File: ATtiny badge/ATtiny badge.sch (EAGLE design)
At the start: 4 parts, among them IC1 TINY13-20SSU

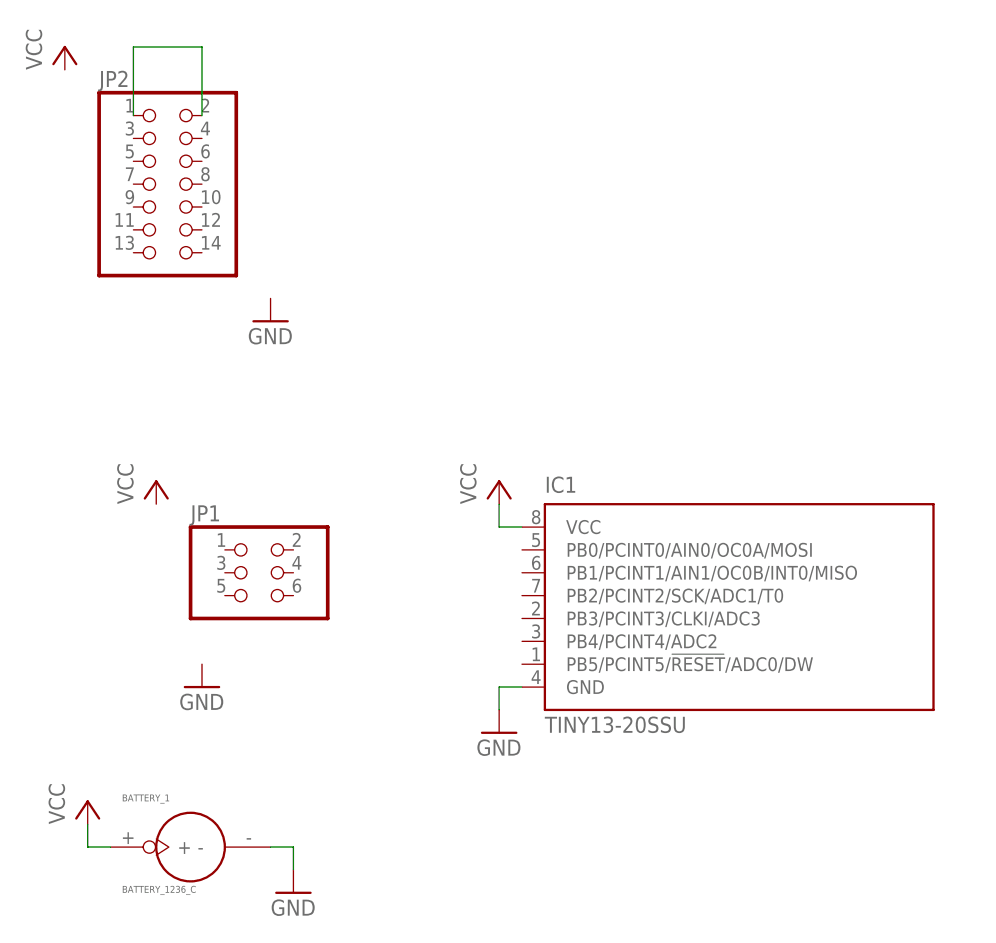
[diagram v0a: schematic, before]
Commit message: new badges
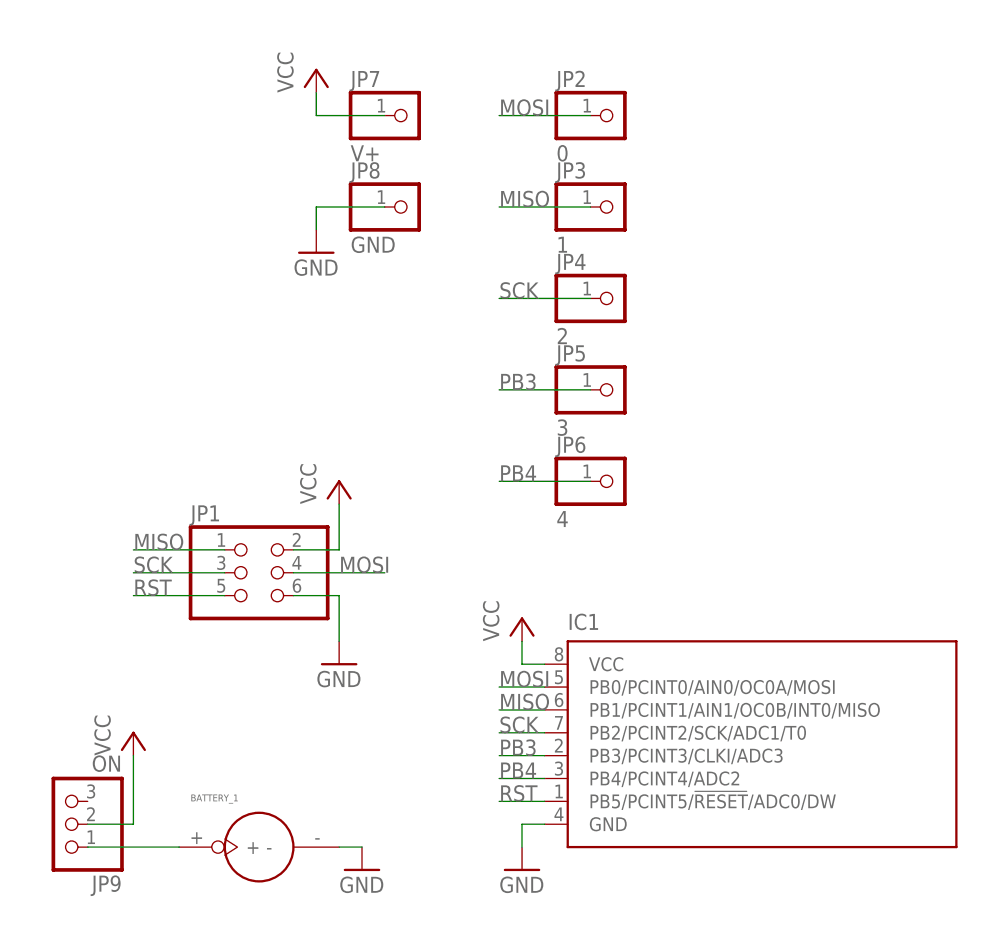
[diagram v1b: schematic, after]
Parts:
- added JP3: 1, pinhead:PINHD-1X1
- added JP4: 2, pinhead:PINHD-1X1
- added JP5: 3, pinhead:PINHD-1X1
- added JP6: 4, pinhead:PINHD-1X1
- added JP7: V+, pinhead:PINHD-1X1
- added JP8: GND, pinhead:PINHD-1X1
- added JP9: ON, pinhead:PINHD-1X3
- IC1: value TINY13-20SSU -> TINY13-20SU; device atmel:TINY13-20SSU -> atmel:TINY13-20SU
- JP2: value (none) -> 0; device pinhead:PINHD-2X7 -> pinhead:PINHD-1X1
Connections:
- new net MISO: IC1.PB1/PCINT1/AIN1/OC0B/INT0/MISO, JP1.1, JP3.1
- new net MOSI: IC1.PB0/PCINT0/AIN0/OC0A/MOSI, JP1.4, JP2.1
- new net PB3: IC1.PB3/PCINT3/CLKI/ADC3, JP5.1
- new net PB4: IC1.PB4/PCINT4/ADC2, JP6.1
- new net RST: IC1.PB5/PCINT5/!RESET!/ADC0/DW, JP1.5
- new net SCK: IC1.PB2/PCINT2/SCK/ADC1/T0, JP1.3, JP4.1
- net GND: now also JP1.6, JP8.1
- net N$1: now also BATTERY_1.+, JP9.1; no longer JP2.1, JP2.2
- net VCC: now also JP1.2, JP7.1, JP9.2; no longer BATTERY_1.+
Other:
- moved on the sheet: BATTERY_1, IC1
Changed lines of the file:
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@@
 </classes>
 <parts>
-<part name="BATTERY_1" library="Itead_BP_110825.lbr" deviceset="BATTERY_1236_C" device=""/>
-<part name="IC1" library="atmel" deviceset="TINY13" device="SSU" technology="-20"/>
+<part name="BATTERY_1" library="Itead_BP_110825.lbr" deviceset="BATTERY_1236_C" device="" value=""/>
+<part name="IC1" library="atmel" deviceset="TINY13" device="SU" technology="-20" value=""/>
 <part name="JP1" library="pinhead" deviceset="PINHD-2X3" device=""/>
-<part name="JP2" library="pinhead" deviceset="PINHD-2X7" device=""/>
 <part name="GND1" library="supply1" deviceset="GND" device=""/>
 <part name="GND2" library="supply1" deviceset="GND" device=""/>
@@
 <part name="P+3" library="supply1" deviceset="VCC" device=""/>
 <part name="P+4" library="supply1" deviceset="VCC" device=""/>
+<part name="JP2" library="pinhead" deviceset="PINHD-1X1" device="" value="0  "/>
+<part name="JP3" library="pinhead" deviceset="PINHD-1X1" device="" value="1  "/>
+<part name="JP4" library="pinhead" deviceset="PINHD-1X1" device="" value="2  "/>
+<part name="JP5" library="pinhead" deviceset="PINHD-1X1" device="" value="3  "/>
+<part name="JP6" library="pinhead" deviceset="PINHD-1X1" device="" value="4  "/>
+<part name="JP7" library="pinhead" deviceset="PINHD-1X1" device="" value="V+"/>
+<part name="JP8" library="pinhead" deviceset="PINHD-1X1" device="" value="GND"/>
+<part name="JP9" library="pinhead" deviceset="PINHD-1X3" device="" value="ON"/>
 </parts>
 <sheets>
@@
 </plain>
 <instances>
-<instance part="BATTERY_1" gate="G$1" x="16.51" y="7.62"/>
-<instance part="IC1" gate="G$1" x="73.66" y="30.48"/>
+<instance part="BATTERY_1" gate="G$1" x="24.13" y="7.62"/>
+<instance part="IC1" gate="G$1" x="76.2" y="15.24"/>
 <instance part="JP1" gate="A" x="22.86" y="38.1"/>
-<instance part="JP2" gate="A" x="12.7" y="81.28"/>
-<instance part="GND1" gate="1" x="27.94" y="2.54"/>
-<instance part="GND2" gate="1" x="50.8" y="20.32"/>
-<instance part="GND3" gate="1" x="25.4" y="66.04"/>
-<instance part="GND4" gate="1" x="17.78" y="25.4"/>
-<instance part="P+1" gate="VCC" x="5.08" y="12.7"/>
-<instance part="P+2" gate="VCC" x="12.7" y="48.26"/>
-<instance part="P+3" gate="VCC" x="50.8" y="48.26"/>
-<instance part="P+4" gate="VCC" x="2.54" y="96.52"/>
+<instance part="GND1" gate="1" x="35.56" y="5.08"/>
+<instance part="GND2" gate="1" x="53.34" y="5.08"/>
+<instance part="GND3" gate="1" x="30.48" y="73.66"/>
+<instance part="GND4" gate="1" x="33.02" y="27.94"/>
+<instance part="P+1" gate="VCC" x="10.16" y="20.32"/>
+<instance part="P+2" gate="VCC" x="33.02" y="48.26"/>
+<instance part="P+3" gate="VCC" x="53.34" y="33.02"/>
+<instance part="P+4" gate="VCC" x="30.48" y="93.98"/>
+<instance part="JP2" gate="G$1" x="63.5" y="88.9"/>
+<instance part="JP3" gate="G$1" x="63.5" y="78.74"/>
+<instance part="JP4" gate="G$1" x="63.5" y="68.58"/>
+<instance part="JP5" gate="G$1" x="63.5" y="58.42"/>
+<instance part="JP6" gate="G$1" x="63.5" y="48.26"/>
+<instance part="JP7" gate="G$1" x="40.64" y="88.9"/>
+<instance part="JP8" gate="G$1" x="40.64" y="78.74"/>
+<instance part="JP9" gate="A" x="2.54" y="10.16" rot="R180"/>
 </instances>
 <busses>
@@
 <pinref part="BATTERY_1" gate="G$1" pin="-"/>
 <pinref part="GND1" gate="1" pin="GND"/>
-<wire x1="25.4" y1="7.62" x2="27.94" y2="7.62" width="0.1524" layer="91"/>
-<wire x1="27.94" y1="7.62" x2="27.94" y2="5.08" width="0.1524" layer="91"/>
+<wire x1="33.02" y1="7.62" x2="35.56" y2="7.62" width="0.1524" layer="91"/>
 </segment>
 <segment>
 <pinref part="IC1" gate="G$1" pin="GND"/>
 <pinref part="GND2" gate="1" pin="GND"/>
-<wire x1="53.34" y1="25.4" x2="50.8" y2="25.4" width="0.1524" layer="91"/>
-<wire x1="50.8" y1="25.4" x2="50.8" y2="22.86" width="0.1524" layer="91"/>
+<wire x1="55.88" y1="10.16" x2="53.34" y2="10.16" width="0.1524" layer="91"/>
+<wire x1="53.34" y1="10.16" x2="53.34" y2="7.62" width="0.1524" layer="91"/>
+</segment>
+<segment>
+<pinref part="GND3" gate="1" pin="GND"/>
+<pinref part="JP8" gate="G$1" pin="1"/>
+<wire x1="30.48" y1="76.2" x2="30.48" y2="78.74" width="0.1524" layer="91"/>
+<wire x1="30.48" y1="78.74" x2="38.1" y2="78.74" width="0.1524" layer="91"/>
+</segment>
+<segment>
+<pinref part="JP1" gate="A" pin="6"/>
+<wire x1="27.94" y1="35.56" x2="33.02" y2="35.56" width="0.1524" layer="91"/>
+<wire x1="33.02" y1="35.56" x2="33.02" y2="30.48" width="0.1524" layer="91"/>
+<pinref part="GND4" gate="1" pin="GND"/>
 </segment>
 </net>
 <net name="VCC" class="0">
 <segment>
-<pinref part="BATTERY_1" gate="G$1" pin="+"/>
-<pinref part="P+1" gate="VCC" pin="VCC"/>
-<wire x1="7.62" y1="7.62" x2="5.08" y2="7.62" width="0.1524" layer="91"/>
-<wire x1="5.08" y1="7.62" x2="5.08" y2="10.16" width="0.1524" layer="91"/>
+<pinref part="IC1" gate="G$1" pin="VCC"/>
+<pinref part="P+3" gate="VCC" pin="VCC"/>
+<wire x1="55.88" y1="27.94" x2="53.34" y2="27.94" width="0.1524" layer="91"/>
+<wire x1="53.34" y1="27.94" x2="53.34" y2="30.48" width="0.1524" layer="91"/>
 </segment>
 <segment>
-<pinref part="IC1" gate="G$1" pin="VCC"/>
-<pinref part="P+3" gate="VCC" pin="VCC"/>
-<wire x1="53.34" y1="43.18" x2="50.8" y2="43.18" width="0.1524" layer="91"/>
-<wire x1="50.8" y1="43.18" x2="50.8" y2="45.72" width="0.1524" layer="91"/>
+<pinref part="P+4" gate="VCC" pin="VCC"/>
+<pinref part="JP7" gate="G$1" pin="1"/>
+<wire x1="30.48" y1="91.44" x2="30.48" y2="88.9" width="0.1524" layer="91"/>
+<wire x1="30.48" y1="88.9" x2="38.1" y2="88.9" width="0.1524" layer="91"/>
+</segment>
+<segment>
+<pinref part="P+2" gate="VCC" pin="VCC"/>
+<wire x1="33.02" y1="45.72" x2="33.02" y2="40.64" width="0.1524" layer="91"/>
+<pinref part="JP1" gate="A" pin="2"/>
+<wire x1="33.02" y1="40.64" x2="27.94" y2="40.64" width="0.1524" layer="91"/>
+</segment>
+<segment>
+<pinref part="JP9" gate="A" pin="2"/>
+<pinref part="P+1" gate="VCC" pin="VCC"/>
+<wire x1="5.08" y1="10.16" x2="10.16" y2="10.16" width="0.1524" layer="91"/>
+<wire x1="10.16" y1="10.16" x2="10.16" y2="17.78" width="0.1524" layer="91"/>
+</segment>
+</net>
+<net name="MISO" class="0">
+<segment>
+<pinref part="JP1" gate="A" pin="1"/>
+<wire x1="20.32" y1="40.64" x2="10.16" y2="40.64" width="0.1524" layer="91"/>
+<label x="10.16" y="40.64" size="1.778" layer="95"/>
+</segment>
+<segment>
+<pinref part="IC1" gate="G$1" pin="PB1/PCINT1/AIN1/OC0B/INT0/MISO"/>
+<wire x1="55.88" y1="22.86" x2="50.8" y2="22.86" width="0.1524" layer="91"/>
+<label x="50.8" y="22.86" size="1.778" layer="95"/>
+</segment>
+<segment>
+<pinref part="JP3" gate="G$1" pin="1"/>
+<wire x1="60.96" y1="78.74" x2="50.8" y2="78.74" width="0.1524" layer="91"/>
+<label x="50.8" y="78.74" size="1.778" layer="95"/>
+</segment>
+</net>
+<net name="SCK" class="0">
+<segment>
+<pinref part="JP1" gate="A" pin="3"/>
+<wire x1="20.32" y1="38.1" x2="10.16" y2="38.1" width="0.1524" layer="91"/>
+<label x="10.16" y="38.1" size="1.778" layer="95"/>
+</segment>
+<segment>
+<pinref part="IC1" gate="G$1" pin="PB2/PCINT2/SCK/ADC1/T0"/>
+<wire x1="50.8" y1="20.32" x2="55.88" y2="20.32" width="0.1524" layer="91"/>
+<label x="50.8" y="20.32" size="1.778" layer="95"/>
+</segment>
+<segment>
+<pinref part="JP4" gate="G$1" pin="1"/>
+<wire x1="60.96" y1="68.58" x2="50.8" y2="68.58" width="0.1524" layer="91"/>
+<label x="50.8" y="68.58" size="1.778" layer="95"/>
+</segment>
+</net>
+<net name="RST" class="0">
+<segment>
+<pinref part="JP1" gate="A" pin="5"/>
+<wire x1="20.32" y1="35.56" x2="10.16" y2="35.56" width="0.1524" layer="91"/>
+<label x="10.16" y="35.56" size="1.778" layer="95"/>
+</segment>
+<segment>
+<pinref part="IC1" gate="G$1" pin="PB5/PCINT5/!RESET!/ADC0/DW"/>
+<wire x1="50.8" y1="12.7" x2="55.88" y2="12.7" width="0.1524" layer="91"/>
+<label x="50.8" y="12.7" size="1.778" layer="95"/>
+</segment>
+</net>
+<net name="MOSI" class="0">
+<segment>
+<pinref part="JP1" gate="A" pin="4"/>
+<wire x1="27.94" y1="38.1" x2="38.1" y2="38.1" width="0.1524" layer="91"/>
+<label x="33.02" y="38.1" size="1.778" layer="95"/>
+</segment>
+<segment>
+<pinref part="IC1" gate="G$1" pin="PB0/PCINT0/AIN0/OC0A/MOSI"/>
+<wire x1="50.8" y1="25.4" x2="55.88" y2="25.4" width="0.1524" layer="91"/>
+<label x="50.8" y="25.4" size="1.778" layer="95"/>
+</segment>
+<segment>
+<pinref part="JP2" gate="G$1" pin="1"/>
+<wire x1="60.96" y1="88.9" x2="50.8" y2="88.9" width="0.1524" layer="91"/>
+<label x="50.8" y="88.9" size="1.778" layer="95"/>
+</segment>
+</net>
+<net name="PB3" class="0">
+<segment>
+<pinref part="IC1" gate="G$1" pin="PB3/PCINT3/CLKI/ADC3"/>
+<wire x1="50.8" y1="17.78" x2="55.88" y2="17.78" width="0.1524" layer="91"/>
+<label x="50.8" y="17.78" size="1.778" layer="95"/>
+</segment>
+<segment>
+<pinref part="JP5" gate="G$1" pin="1"/>
+<wire x1="60.96" y1="58.42" x2="50.8" y2="58.42" width="0.1524" layer="91"/>
+<label x="50.8" y="58.42" size="1.778" layer="95"/>
+</segment>
+</net>
+<net name="PB4" class="0">
+<segment>
+<pinref part="IC1" gate="G$1" pin="PB4/PCINT4/ADC2"/>
+<wire x1="50.8" y1="15.24" x2="55.88" y2="15.24" width="0.1524" layer="91"/>
+<label x="50.8" y="15.24" size="1.778" layer="95"/>
+</segment>
+<segment>
+<pinref part="JP6" gate="G$1" pin="1"/>
+<wire x1="60.96" y1="48.26" x2="50.8" y2="48.26" width="0.1524" layer="91"/>
+<label x="50.8" y="48.26" size="1.778" layer="95"/>
 </segment>
 </net>
 <net name="N$1" class="0">
 <segment>
-<pinref part="JP2" gate="A" pin="1"/>
-<wire x1="10.16" y1="88.9" x2="10.16" y2="96.52" width="0.1524" layer="91"/>
-<wire x1="10.16" y1="96.52" x2="17.78" y2="96.52" width="0.1524" layer="91"/>
-<pinref part="JP2" gate="A" pin="2"/>
-<wire x1="17.78" y1="96.52" x2="17.78" y2="88.9" width="0.1524" layer="91"/>
+<pinref part="JP9" gate="A" pin="1"/>
+<pinref part="BATTERY_1" gate="G$1" pin="+"/>
+<wire x1="5.08" y1="7.62" x2="15.24" y2="7.62" width="0.1524" layer="91"/>
 </segment>
 </net>

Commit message: renderings + gerbers
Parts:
- JP2: value 0 -> 0
- JP3: value 1 -> 1
- JP4: value 2 -> 2
- JP5: value 3 -> 3
- JP6: value 4 -> 4
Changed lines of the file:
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@@
 <part name="P+3" library="supply1" deviceset="VCC" device=""/>
 <part name="P+4" library="supply1" deviceset="VCC" device=""/>
-<part name="JP2" library="pinhead" deviceset="PINHD-1X1" device="" value="0  "/>
-<part name="JP3" library="pinhead" deviceset="PINHD-1X1" device="" value="1  "/>
-<part name="JP4" library="pinhead" deviceset="PINHD-1X1" device="" value="2  "/>
-<part name="JP5" library="pinhead" deviceset="PINHD-1X1" device="" value="3  "/>
-<part name="JP6" library="pinhead" deviceset="PINHD-1X1" device="" value="4  "/>
+<part name="JP2" library="pinhead" deviceset="PINHD-1X1" device="" value="0"/>
+<part name="JP3" library="pinhead" deviceset="PINHD-1X1" device="" value="1"/>
+<part name="JP4" library="pinhead" deviceset="PINHD-1X1" device="" value="2"/>
+<part name="JP5" library="pinhead" deviceset="PINHD-1X1" device="" value="3"/>
+<part name="JP6" library="pinhead" deviceset="PINHD-1X1" device="" value="4"/>
 <part name="JP7" library="pinhead" deviceset="PINHD-1X1" device="" value="V+"/>
 <part name="JP8" library="pinhead" deviceset="PINHD-1X1" device="" value="GND"/>
